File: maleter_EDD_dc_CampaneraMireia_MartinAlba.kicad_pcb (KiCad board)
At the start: 2 copper layers, 85 x 68.5 mm, 66 parts, among them J1 Conn_01x02_Pin, J2 DE9_Pins, J3 DE9_Pins, J4 Conn_01x05_Pin, M1 Motor_DC_ALT, Q1 IRLZ44N, SW1 SW_DPST_x2, SW2 SW_DPST_x2, SW3 SW_DPST_x2, SW5 SW_Push, U1 LM2596S-5, U2 LM1117DT-3.3, U3 PIC24HJ128GP502, U4 MCP2551-I-SN, U5 DRV8871DDA, U7 VL53L0CXV0DH1, U8 MAX3232, U9 LM358, Y1 8MHz

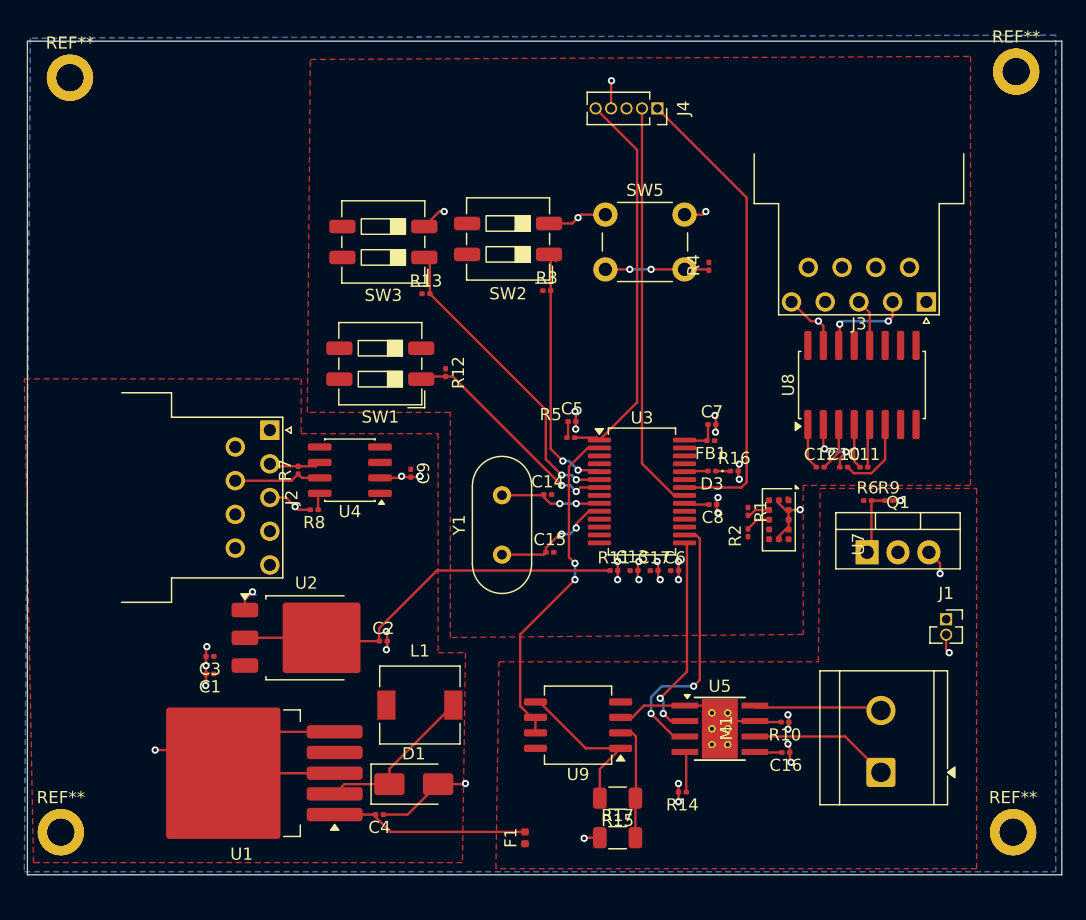
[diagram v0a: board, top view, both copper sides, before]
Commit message: Actualització projecte a classe
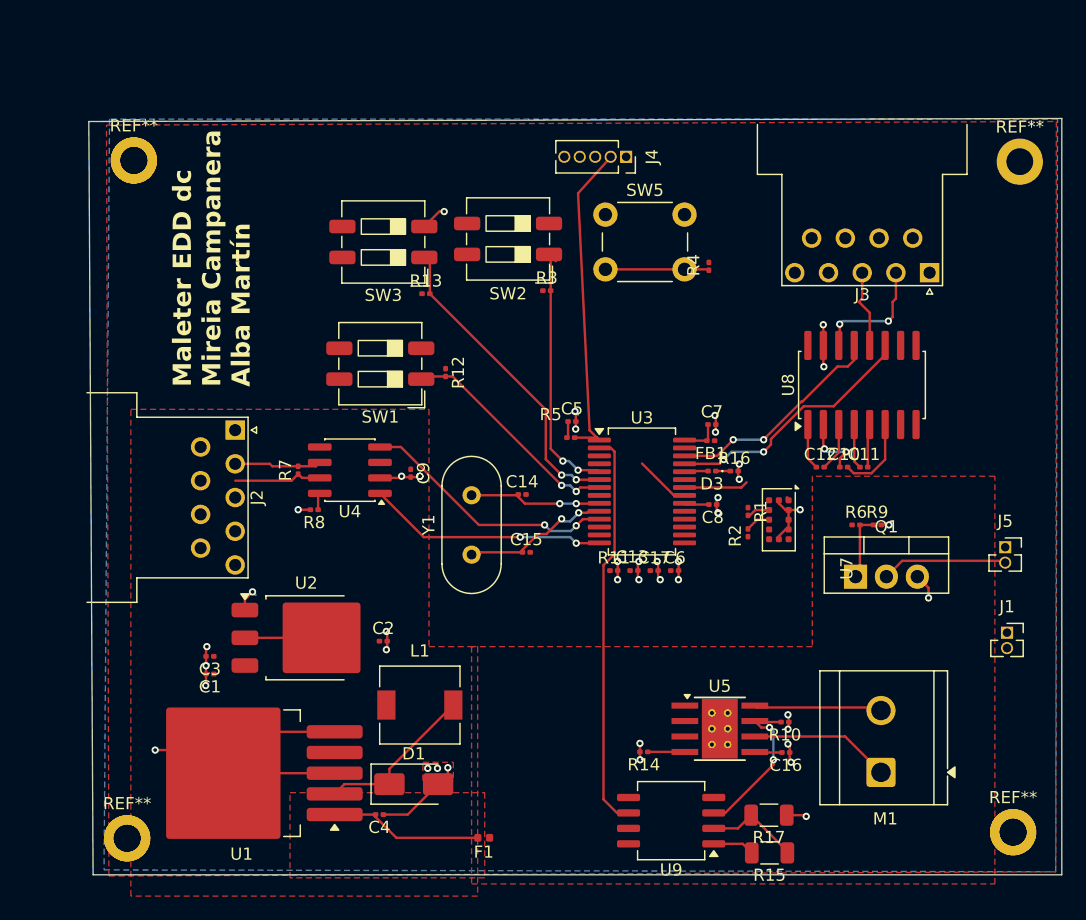
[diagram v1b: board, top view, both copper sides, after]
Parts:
- removed the ? at (175.8, 83.8)
- added J5: Conn_01x02_Pin, Connector_PinSocket_1.27mm:PinSocket_1x02_P1.27mm_Vertical, F.Cu at (174.8, 122.8)
- moved R15 13.3 mm to (155.5, 147.9)
- moved R17 12.6 mm to (155.4, 144.8), turned to 180 degrees
- moved U9 11.0 mm to (147.4, 145.3)
- moved ? 8.59 mm to (103.2, 91.0)
- moved REF** 8.59 mm to (103.2, 91.0)
- moved REF** 7.41 mm to (176.1, 91.2)
- moved ? 5.47 mm to (102.7, 146.8)
- moved REF** 5.47 mm to (102.7, 146.8)
- moved J1 5.12 mm to (175.0, 129.8)
- moved J4 4.74 mm to (143.7, 90.8)
- moved R14 4.57 mm to (145.2, 139.7)
- moved F1 3.39 mm to (132.0, 146.7), turned to 180 degrees
- moved J2 2.85 mm to (111.6, 113.2)
- moved Y1 2.50 mm to (131.0, 123.4)
- moved J3 2.42 mm to (168.6, 100.3)
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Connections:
- net Net-(D1-K) renamed /ALIMENTACIO I MOTOR/Vout
- net Net-(D3-A) renamed /CONTROL UNIT/LED
- net Net-(D3-K) renamed /CONTROL UNIT/R_LED
- net Net-(M1-+) renamed /ALIMENTACIO I MOTOR/OUT1
- net Net-(M1--) renamed /ALIMENTACIO I MOTOR/OUT2
- net Net-(U1-VIN) renamed /ALIMENTACIO I MOTOR/Vin
- net Net-(U3-AVDD) renamed /CONTROL UNIT/AVDD
- net Net-(U3-OSC1) renamed /CONTROL UNIT/OSC1
- net Net-(U3-OSC2) renamed /CONTROL UNIT/OSC2
- net Net-(U3-VCAP) renamed /CONTROL UNIT/VCAP
- net Net-(U4-Rs) renamed /CONTROL UNIT/Rs
- net Net-(U5-ILIM) renamed /ALIMENTACIO I MOTOR/ILIM
- net Net-(U8-C1+) renamed /CONTROL UNIT/C1+
- net Net-(U8-C1-) renamed /CONTROL UNIT/C1-
- net Net-(U8-C2+) renamed /CONTROL UNIT/C2+
- net Net-(U8-C2-) renamed /CONTROL UNIT/C2-
- net Net-(U8-VS+) renamed /CONTROL UNIT/VS+
- net Net-(U8-VS-) renamed /CONTROL UNIT/VS-
- C5 pad 1: Net-(C5-Pad1) -> MCLR
- Q1 pad 1: Net-(Q1-G) -> CV
- Q1 pad 2: +12V -> /CONTROL UNIT/Conn_calefactor
- R10 pad 2: Net-(U9A-+) -> /ALIMENTACIO I MOTOR/PGND
- R4 pad 2: Net-(C5-Pad1) -> MCLR
- R5 pad 1: Net-(C5-Pad1) -> MCLR
- R6 pad 2: Net-(Q1-G) -> CV
- R9 pad 1: Net-(Q1-G) -> CV
- SW5 pad 2: Net-(C5-Pad1) -> MCLR
- U3 pad 11: unconnected-(U3-RB4-Pad11) -> RX_CAN
- U3 pad 14: unconnected-(U3-RB5-Pad14) -> TX_CAN
- U3 pad 25: unconnected-(U3-RB14-Pad25) -> TX_USART
- U3 pad 26: unconnected-(U3-RB15-Pad26) -> RX_USART
- U5 pad 1: Net-(U9A-+) -> GND
- U5 pad 7: Net-(U9A-+) -> /ALIMENTACIO I MOTOR/PGND
- U5 pad 9: Net-(U9A-+) -> GND
- U9 pad 3: Net-(U9A-+) -> /ALIMENTACIO I MOTOR/PGND
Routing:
- net /CONTROL UNIT/PGC: track 39.0 -> 5.28 mm
- net /CONTROL UNIT/PGD: track 33.8 -> 4.58 mm
- net 3.3V: track 33.2 -> 6.73 mm
- net PWM: track 22.5 -> 0.89 mm, vias 2 -> 0
- net RX_CAN: track 0.00 -> 21.3 mm, vias 0 -> 2
- net TX_USART: track 0.00 -> 21.2 mm, vias 0 -> 2
- net TX_CAN: track 0.00 -> 19.7 mm, vias 0 -> 2
- net RX_USART: track 0.00 -> 18.5 mm, vias 0 -> 2
- net Direccio: track 17.2 -> 0.00 mm, vias 2 -> 0
- net GND: track 92.2 -> 78.8 mm, vias 44 -> 43
- net /ALIMENTACIO I MOTOR/PGND: track 0.00 -> 13.4 mm, vias 0 -> 2
- net Net-(U9A-+): track 12.8 -> 0.00 mm
- net /CONTROL UNIT/Conn_calefactor: track 0.00 -> 10.4 mm
- net Net-(C5-Pad1): track 10.0 -> 0.00 mm, vias 2 -> 0
- net /ALIMENTACIO I MOTOR/outamp: track 13.4 -> 3.43 mm
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- added copper zone on F.Cu, net GND
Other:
- board size 85 x 68.5 mm -> 80 x 62.2 mm
- board text added: "Maleter EDD dc Mireia Campanera Alba Martín"
